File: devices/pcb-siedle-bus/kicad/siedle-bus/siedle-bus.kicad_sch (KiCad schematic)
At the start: 34 parts, among them J1 Conn_01x02, Q1 IRLML0030, Q2 BC807, Q3 BC807, Q4 IRLML0030, Q5 IRLML0030, SW1 RESET, SW2 BOOT, U2 ESP32-WROOM-32

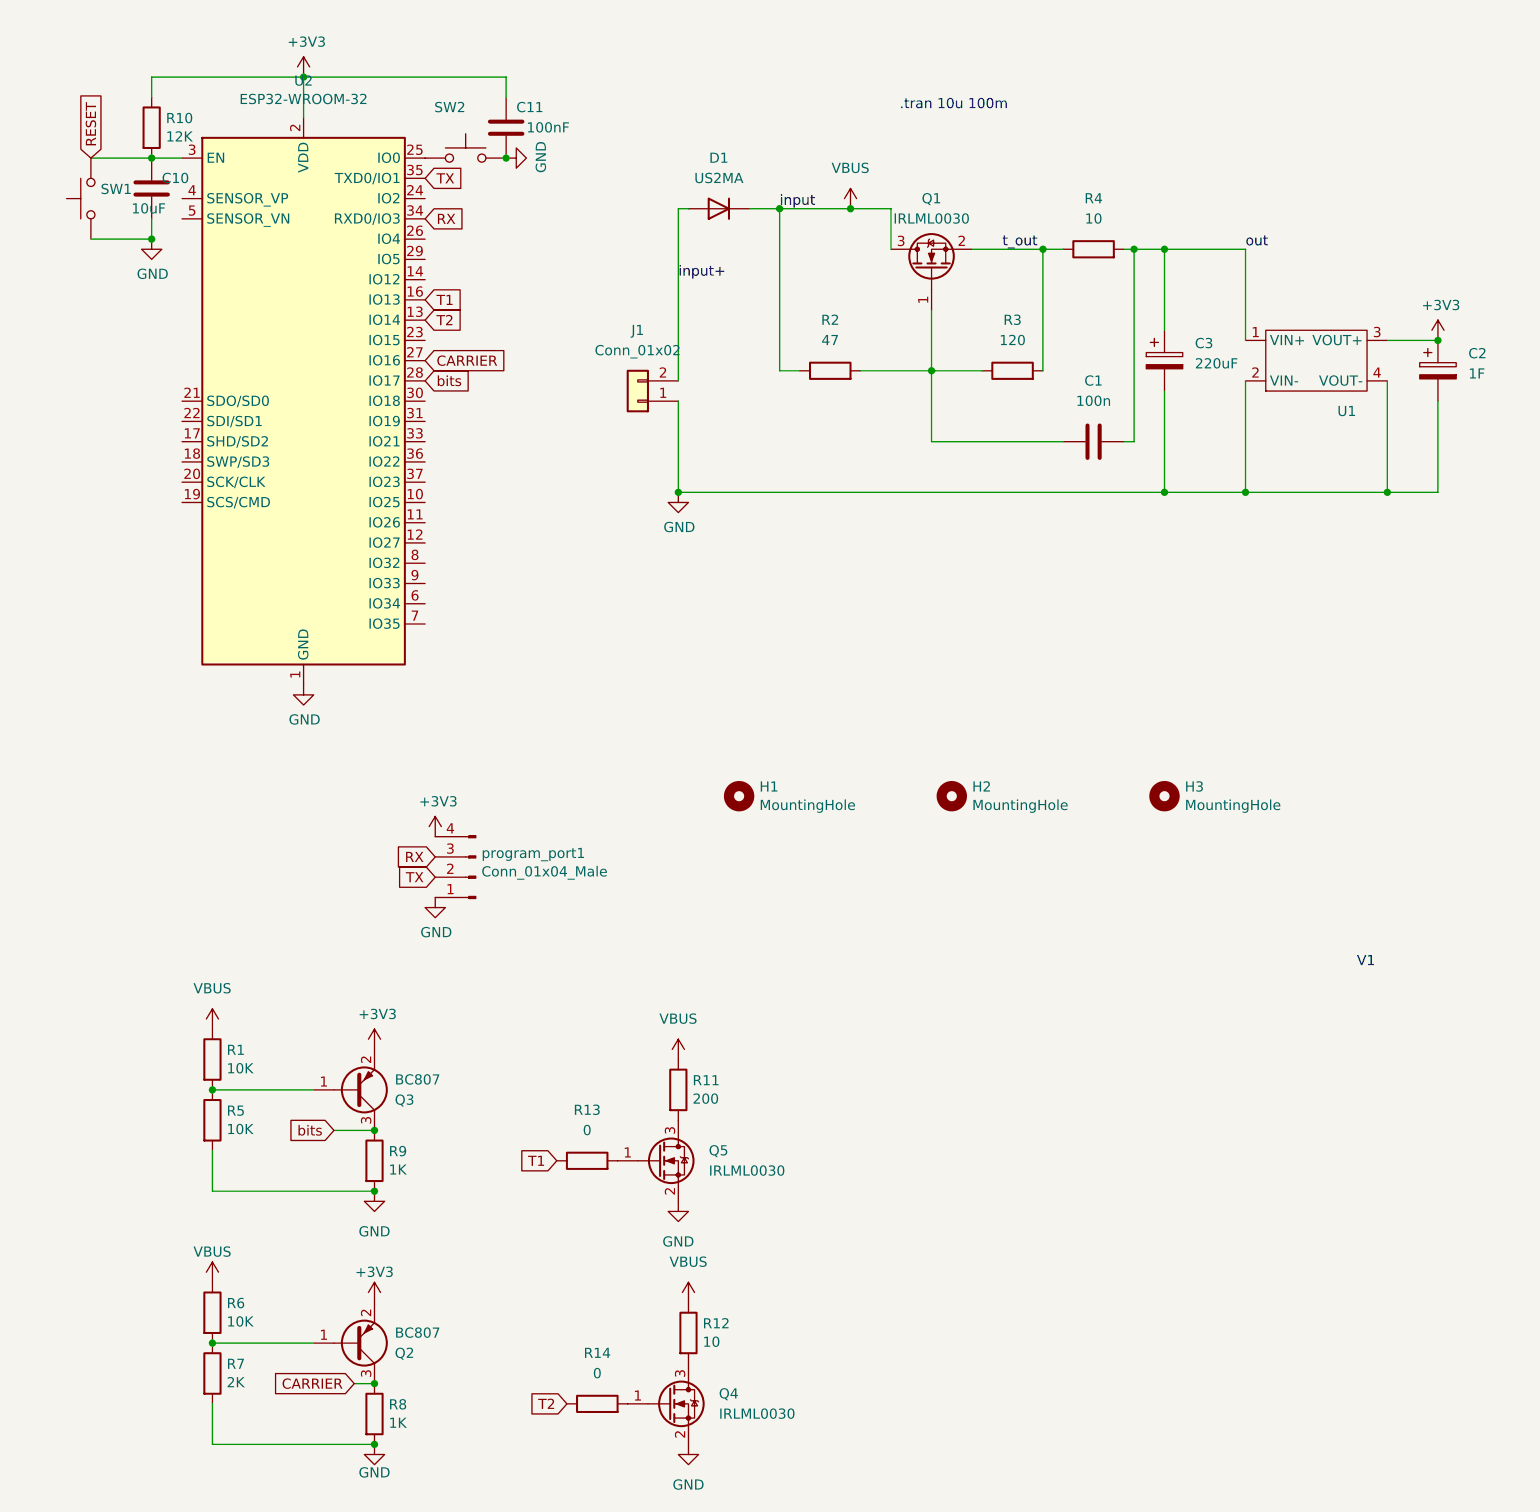
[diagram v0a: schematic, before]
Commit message: progress with siedle
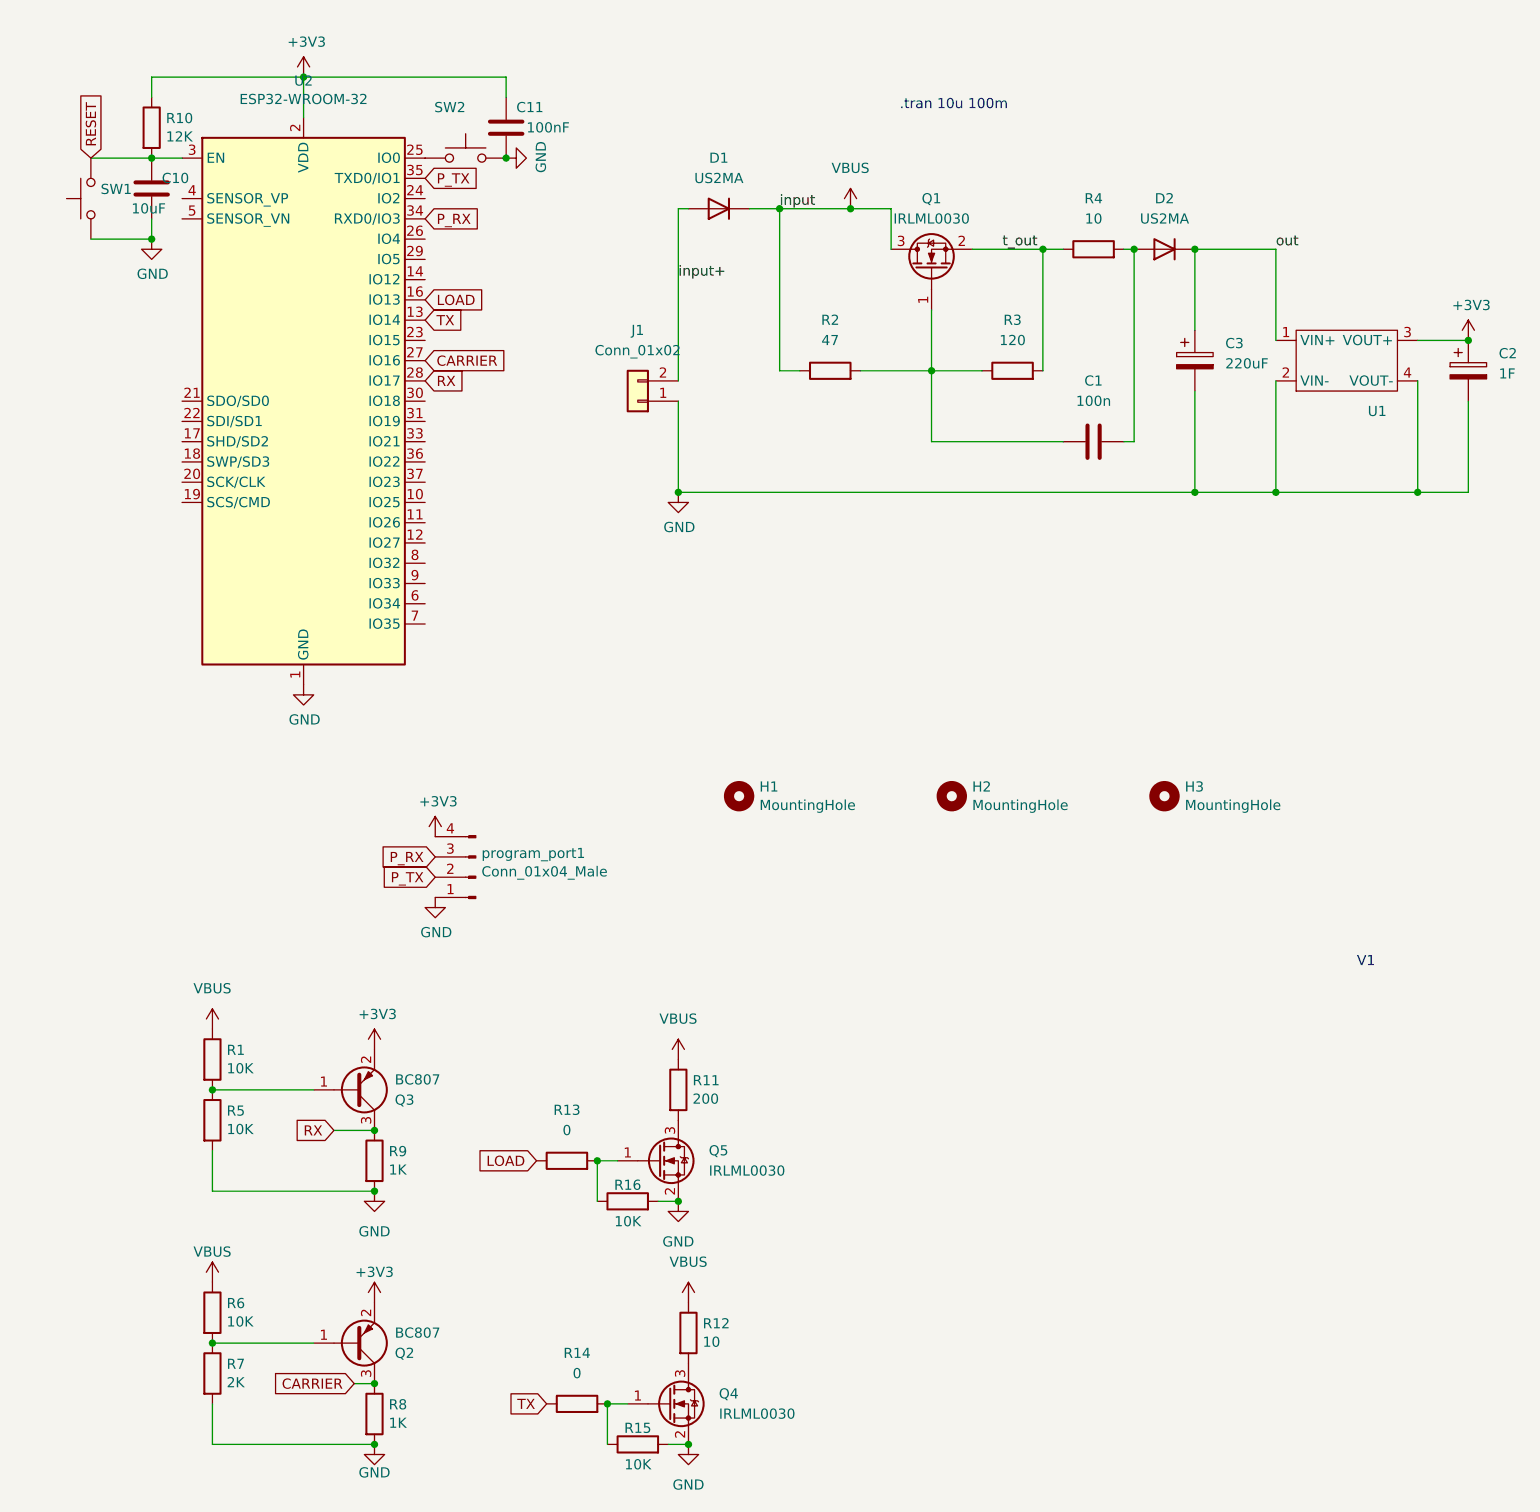
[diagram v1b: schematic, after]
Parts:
- added D2: US2MA, Diode_SMD:D_SMA, symbol Diode:US2MA
- added R15, R16: 10K, Resistor_SMD:R_0805_2012Metric, symbol Device:R
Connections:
- net T2 is gone; now on net TX: R14.1, U2.13 (IO14)
- net bits is gone; now on net RX: Q3.3 (C), R9.1, U2.28 (IO17)
- net GND: now also R15.2, R16.2
- net RX: no longer U2.34 (RXD0/IO3), program_port1.3 (Pin_3)
- net TX: no longer U2.35 (TXD0/IO1), program_port1.2 (Pin_2)
- net out: now also D2.1 (K); no longer C1.2, R4.2
- net at Q5.1 (G), R13.2: now also R16.1
- net at Q4.1 (G), R14.2: now also R15.1
- net T1 renamed LOAD
- new net: C1.2, D2.2 (A), R4.2
- new net P_RX: U2.34 (RXD0/IO3), program_port1.3 (Pin_3)
- new net P_TX: U2.35 (TXD0/IO1), program_port1.2 (Pin_2)
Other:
- moved on the sheet: C2, C3, R13, R14, U1

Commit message: clean readme
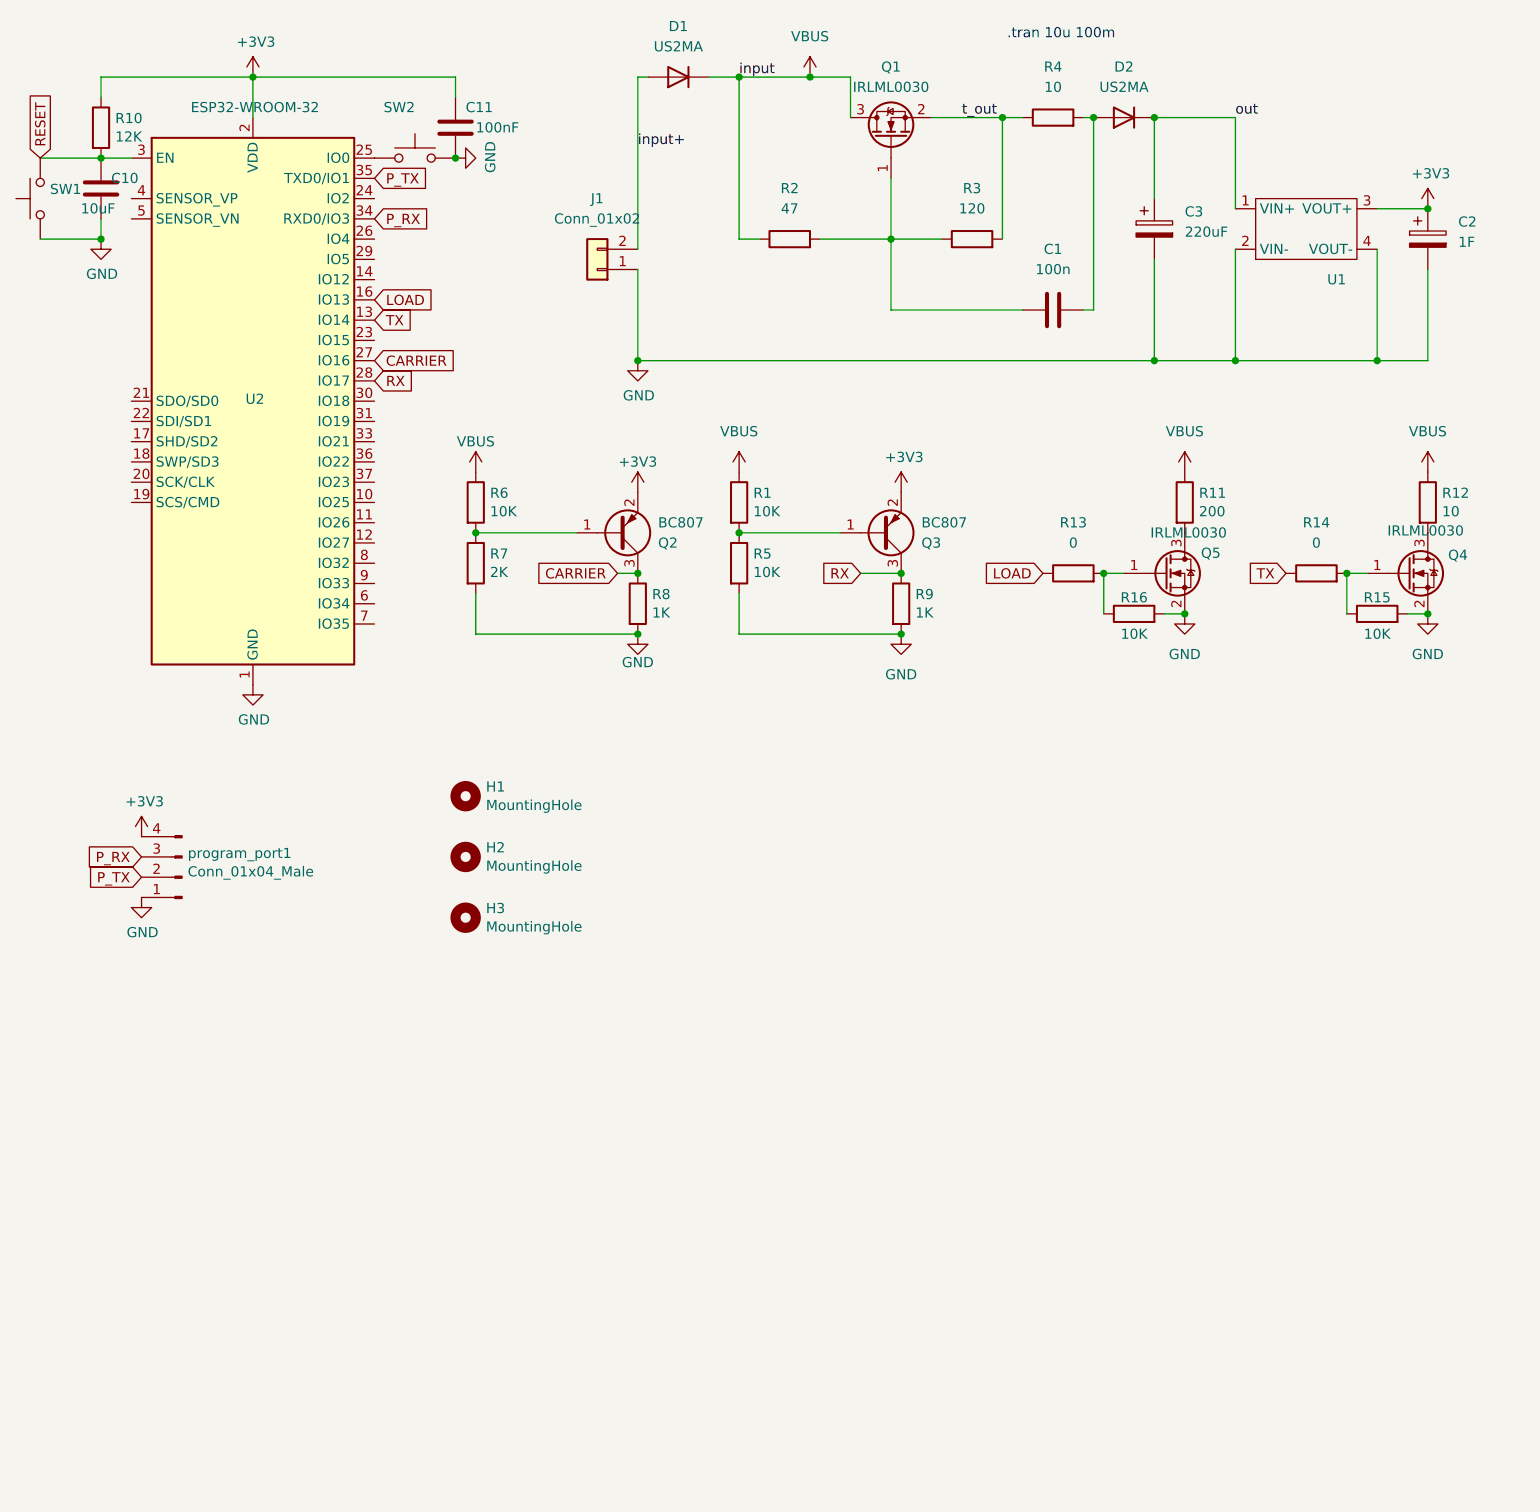
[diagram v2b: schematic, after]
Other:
- note removed: "V1"
- title: (none) -> Siedle In-Home Bus client
- moved on the sheet: C1, C10, C11, C2, C3, D1, D2, H1, H2, H3, J1, Q1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
